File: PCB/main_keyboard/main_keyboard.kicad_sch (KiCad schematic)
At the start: 215 parts, among them J1 Conn_01x05_Pin, J2 Conn_01x04_Pin, SW1 SW_Push, U1 ATmega32U4-A, Y1 Crystal 8MHz

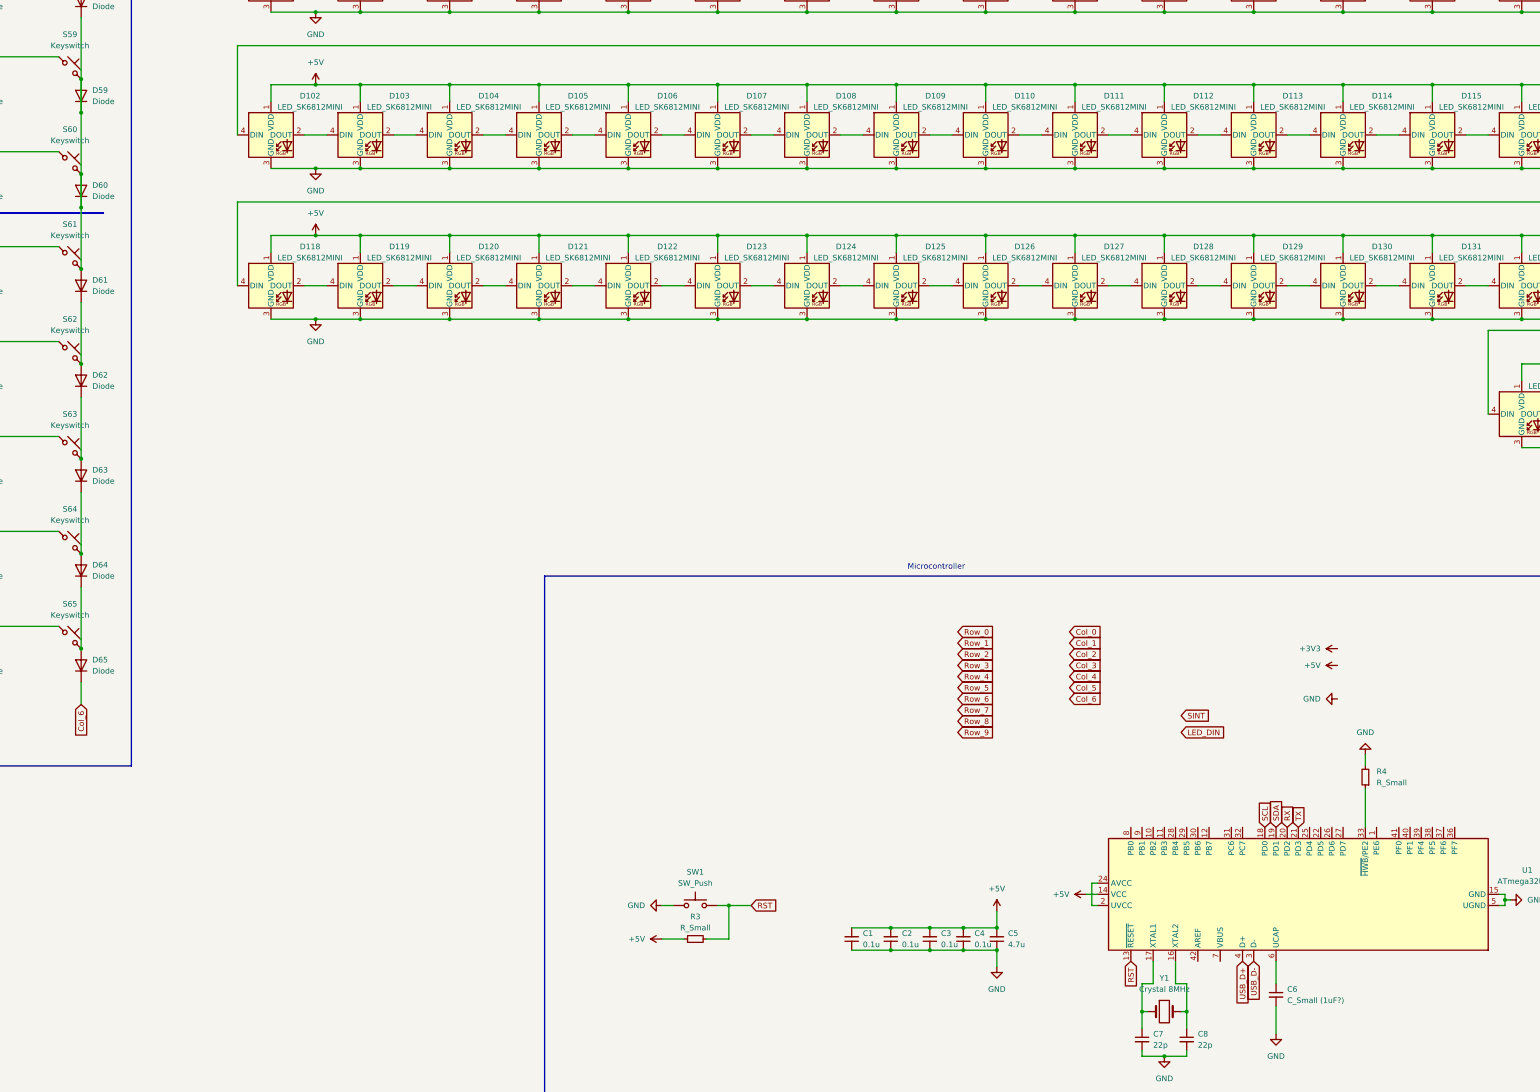
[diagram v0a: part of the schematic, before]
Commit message: First draft Main board
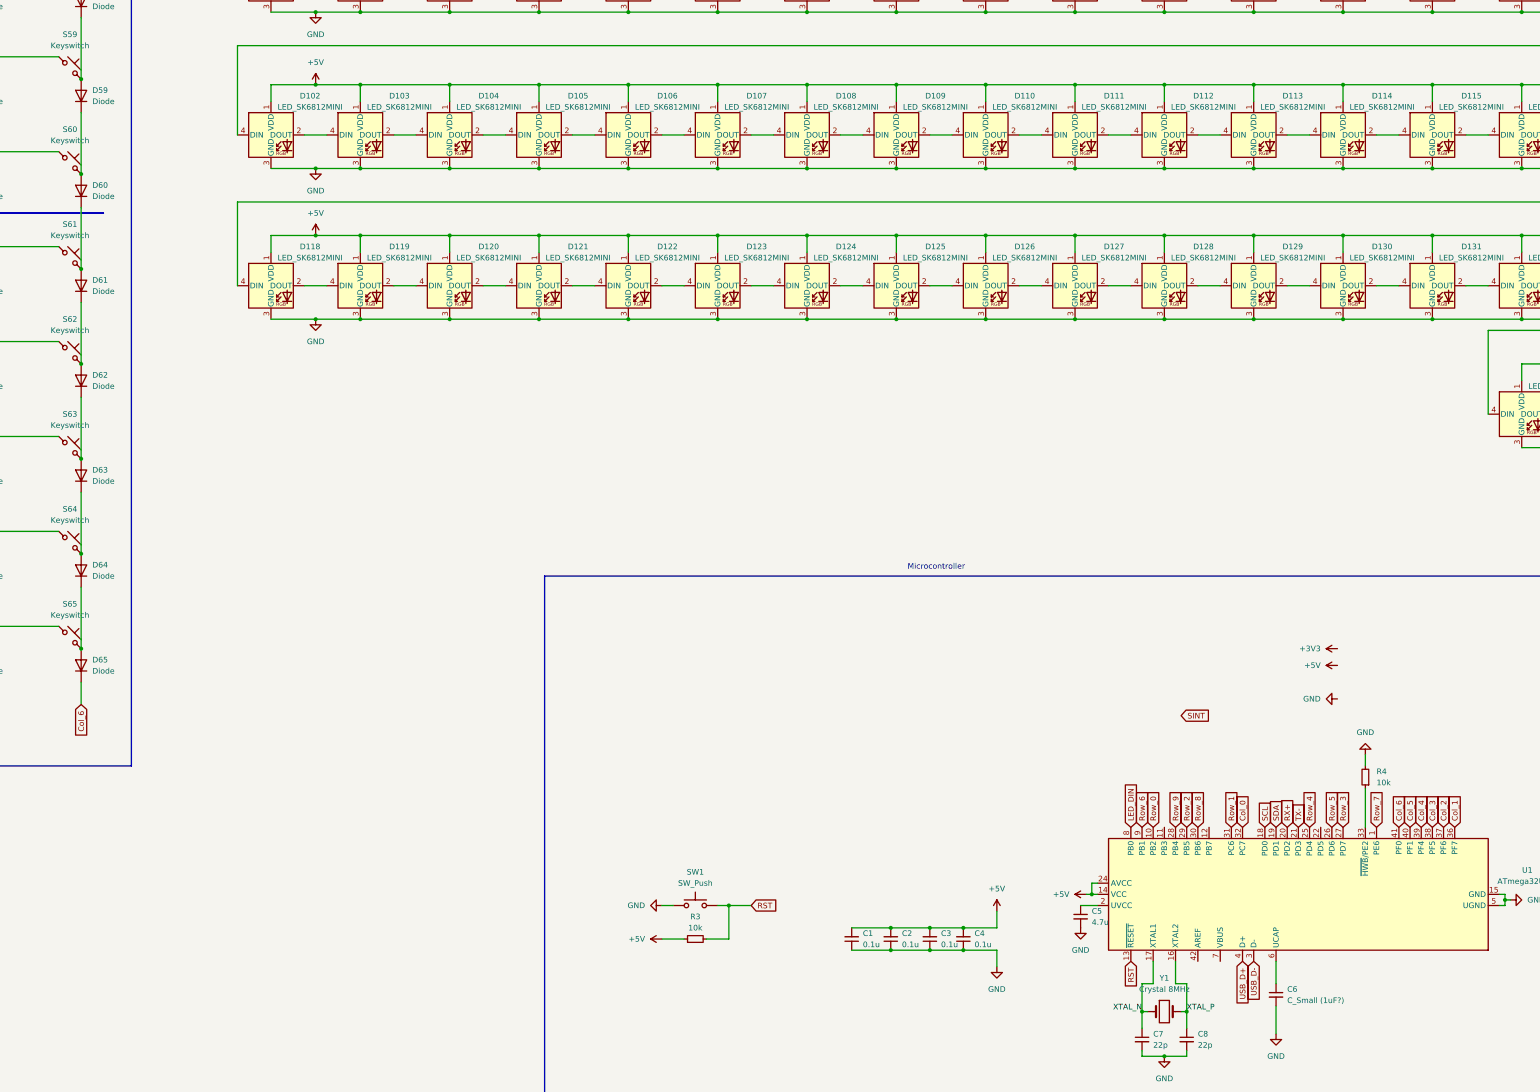
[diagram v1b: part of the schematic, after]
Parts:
- C1, C2, C3, C4, C7, C8: footprint Capacitor_SMD:C_01005_0402Metric_Pad0.57x0.30mm_HandSolder -> Capacitor_SMD:C_0805_2012Metric_Pad1.18x1.45mm_HandSolder
- C5: footprint Capacitor_SMD:C_0201_0603Metric_Pad0.64x0.40mm_HandSolder -> Capacitor_SMD:C_0603_1608Metric_Pad1.08x0.95mm_HandSolder
- C6: footprint (none) -> Capacitor_SMD:C_0603_1608Metric_Pad1.08x0.95mm_HandSolder
- J1: footprint Connector:FanPinHeader_1x03_P2.54mm_Vertical -> Connector_PinHeader_2.54mm:PinHeader_1x05_P2.54mm_Vertical
- J2: footprint (none) -> Connector_JST:JST_EH_S4B-EH_1x04_P2.50mm_Horizontal
- R3, R4: value R_Small -> 10k; footprint (none) -> Resistor_SMD:R_0805_2012Metric_Pad1.20x1.40mm_HandSolder
- SW1: footprint (none) -> Connector_PinHeader_1.00mm:PinHeader_1x02_P1.00mm_Vertical
- Y1: footprint (none) -> Crystal:Crystal_HC18-U_Vertical
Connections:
- net +5V: now also U1.24 (AVCC), U1.44 (AVCC); no longer C5.2
- net Col_0: now also U1.32 (PC7)
- net Col_1: now also U1.36 (PF7)
- net Col_2: now also U1.37 (PF6)
- net Col_3: now also U1.38 (PF5)
- net Col_4: now also U1.39 (PF4)
- net Col_5: now also U1.40 (PF1)
- net Col_6: now also U1.41 (PF0)
- net GND: now also C5.2; no longer C5.1
- net LED_DIN: now also U1.8 (PB0)
- net Row_0: now also U1.10 (PB2)
- net Row_1: now also U1.31 (PC6)
- net Row_2: now also U1.29 (PB5)
- net Row_3: now also U1.27 (PD7)
- net Row_4: now also U1.25 (PD4)
- net Row_5: now also U1.26 (PD6)
- net Row_6: now also U1.9 (PB1)
- net Row_7: now also U1.1 (PE6)
- net Row_8: now also U1.30 (PB6)
- net Row_9: now also U1.28 (PB4)
- net XTAL_P: now reaches C8.1, U1.16 (XTAL2), Y1.2
- net XTAL_N: now reaches C7.1, U1.17 (XTAL1), Y1.1
- net RX renamed RX+
- net TX renamed TX-
- new net: D58.1 (K), D59.2 (A), S59.2
- new net: D59.1 (K), D60.2 (A), S60.2
- new net: C5.1, U1.2 (UVCC)
- new net: D60.1 (K), D61.2 (A), S61.2
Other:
- moved on the sheet: C5
